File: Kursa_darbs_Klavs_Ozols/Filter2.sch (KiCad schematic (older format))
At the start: 11 parts, among them U1 TL074

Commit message: Shii ir kursa darba 3. iteraacija
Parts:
- C15, C16, C17, C18: footprint (none) -> Capacitors_THT:C_Axial_L5.1mm_D3.1mm_P10.00mm_Horizontal
- R10, R11, R12, R7, R8, R9: footprint (none) -> Resistors_THT:R_Axial_DIN0309_L9.0mm_D3.2mm_P5.08mm_Vertical
- U1: footprint (none) -> TL074:DIL14
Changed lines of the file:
@@
 F 0 "U1" H 3450 2900 50  0000 L CNN
 F 1 "TL074" H 3450 2500 50  0000 L CNN
-F 2 "" H 3400 2800 50  0001 C CNN
+F 2 "TL074:DIL14" H 3400 2800 50  0001 C CNN
 F 3 "" H 3500 2900 50  0001 C CNN
 	3    3450 2700
@@
 F 0 "U1" H 5600 2900 50  0000 L CNN
 F 1 "TL074" H 5600 2500 50  0000 L CNN
-F 2 "" H 5550 2800 50  0001 C CNN
+F 2 "TL074:DIL14" H 5550 2800 50  0001 C CNN
 F 3 "" H 5650 2900 50  0001 C CNN
 	4    5600 2700
@@
 F 0 "R7" V 2380 2800 50  0000 C CNN
 F 1 "6.8 k" V 2300 2800 50  0000 C CNN
-F 2 "" V 2230 2800 50  0001 C CNN
-F 3 "" H 2300 2800 50  0001 C CNN
+F 2 "Resistors_THT:R_Axial_DIN0309_L9.0mm_D3.2mm_P5.08mm_Vertical" V 2230 2800 50  0001 C CNN
+F 3 "https://eu.mouser.com/datasheet/2/219/MOS-16613.pdf" H 2300 2800 50  0001 C CNN
 	1    2300 2800
 	0    1    1    0
@@
 F 0 "R8" V 2630 2550 50  0000 C CNN
 F 1 "5.1 k" V 2550 2550 50  0000 C CNN
-F 2 "" V 2480 2550 50  0001 C CNN
-F 3 "" H 2550 2550 50  0001 C CNN
+F 2 "Resistors_THT:R_Axial_DIN0309_L9.0mm_D3.2mm_P5.08mm_Vertical" V 2480 2550 50  0001 C CNN
+F 3 "https://eu.mouser.com/datasheet/2/219/MOS-16613.pdf" H 2550 2550 50  0001 C CNN
 	1    2550 2550
 	1    0    0    -1
@@
 F 0 "R9" V 3030 3000 50  0000 C CNN
 F 1 "62k" V 2950 3000 50  0000 C CNN
-F 2 "" V 2880 3000 50  0001 C CNN
-F 3 "" H 2950 3000 50  0001 C CNN
+F 2 "Resistors_THT:R_Axial_DIN0309_L9.0mm_D3.2mm_P5.08mm_Vertical" V 2880 3000 50  0001 C CNN
+F 3 "https://eu.mouser.com/datasheet/2/219/MOS-16613.pdf" H 2950 3000 50  0001 C CNN
 	1    2950 3000
 	1    0    0    -1
@@
 F 0 "C18" H 4960 3270 50  0000 L CNN
 F 1 "220 nF" H 4960 3120 50  0000 L CNN
-F 2 "" H 4950 3200 50  0001 C CNN
-F 3 "" H 4950 3200 50  0001 C CNN
+F 2 "Capacitors_THT:C_Axial_L5.1mm_D3.1mm_P10.00mm_Horizontal" H 4950 3200 50  0001 C CNN
+F 3 "https://eu.mouser.com/datasheet/2/212/KEM_C1046_AXIAL_MOLDED_X7R-1145195.pdf" H 4950 3200 50  0001 C CNN
 	1    4950 3200
 	0    1    1    0
@@
 F 0 "C16" H 2760 3320 50  0000 L CNN
 F 1 "220 nF" H 2760 3170 50  0000 L CNN
-F 2 "" H 2750 3250 50  0001 C CNN
-F 3 "" H 2750 3250 50  0001 C CNN
+F 2 "Capacitors_THT:C_Axial_L5.1mm_D3.1mm_P10.00mm_Horizontal" H 2750 3250 50  0001 C CNN
+F 3 "https://eu.mouser.com/datasheet/2/212/KEM_C1046_AXIAL_MOLDED_X7R-1145195.pdf" H 2750 3250 50  0001 C CNN
 	1    2750 3250
 	0    1    1    0
@@
 F 0 "C15" H 2760 2870 50  0000 L CNN
 F 1 "220 nF" H 2760 2720 50  0000 L CNN
-F 2 "" H 2750 2800 50  0001 C CNN
-F 3 "" H 2750 2800 50  0001 C CNN
+F 2 "Capacitors_THT:C_Axial_L5.1mm_D3.1mm_P10.00mm_Horizontal" H 2750 2800 50  0001 C CNN
+F 3 "https://eu.mouser.com/datasheet/2/212/KEM_C1046_AXIAL_MOLDED_X7R-1145195.pdf" H 2750 2800 50  0001 C CNN
 	1    2750 2800
 	0    1    1    0
@@
 F 0 "R10" V 4330 2700 50  0000 C CNN
 F 1 "6.8 k" V 4250 2700 50  0000 C CNN
-F 2 "" V 4180 2700 50  0001 C CNN
-F 3 "" H 4250 2700 50  0001 C CNN
+F 2 "Resistors_THT:R_Axial_DIN0309_L9.0mm_D3.2mm_P5.08mm_Vertical" V 4180 2700 50  0001 C CNN
+F 3 "https://eu.mouser.com/datasheet/2/219/MOS-16613.pdf" H 4250 2700 50  0001 C CNN
 	1    4250 2700
 	0    1    1    0
@@
 F 0 "C17" H 4960 2870 50  0000 L CNN
 F 1 "220 nF" H 4960 2720 50  0000 L CNN
-F 2 "" H 4950 2800 50  0001 C CNN
-F 3 "" H 4950 2800 50  0001 C CNN
+F 2 "Capacitors_THT:C_Axial_L5.1mm_D3.1mm_P10.00mm_Horizontal" H 4950 2800 50  0001 C CNN
+F 3 "https://eu.mouser.com/datasheet/2/212/KEM_C1046_AXIAL_MOLDED_X7R-1145195.pdf" H 4950 2800 50  0001 C CNN
 	1    4950 2800
 	0    1    1    0
@@
 F 0 "R12" V 5280 3000 50  0000 C CNN
 F 1 "62k" V 5200 3000 50  0000 C CNN
-F 2 "" V 5130 3000 50  0001 C CNN
-F 3 "" H 5200 3000 50  0001 C CNN
+F 2 "Resistors_THT:R_Axial_DIN0309_L9.0mm_D3.2mm_P5.08mm_Vertical" V 5130 3000 50  0001 C CNN
+F 3 "https://eu.mouser.com/datasheet/2/219/MOS-16613.pdf" H 5200 3000 50  0001 C CNN
 	1    5200 3000
 	1    0    0    -1
@@
 F 0 "R11" V 4730 2450 50  0000 C CNN
 F 1 "5.1 k" V 4650 2450 50  0000 C CNN
-F 2 "" V 4580 2450 50  0001 C CNN
-F 3 "" H 4650 2450 50  0001 C CNN
+F 2 "Resistors_THT:R_Axial_DIN0309_L9.0mm_D3.2mm_P5.08mm_Vertical" V 4580 2450 50  0001 C CNN
+F 3 "https://eu.mouser.com/datasheet/2/219/MOS-16613.pdf" H 4650 2450 50  0001 C CNN
 	1    4650 2450
 	0    1    1    0

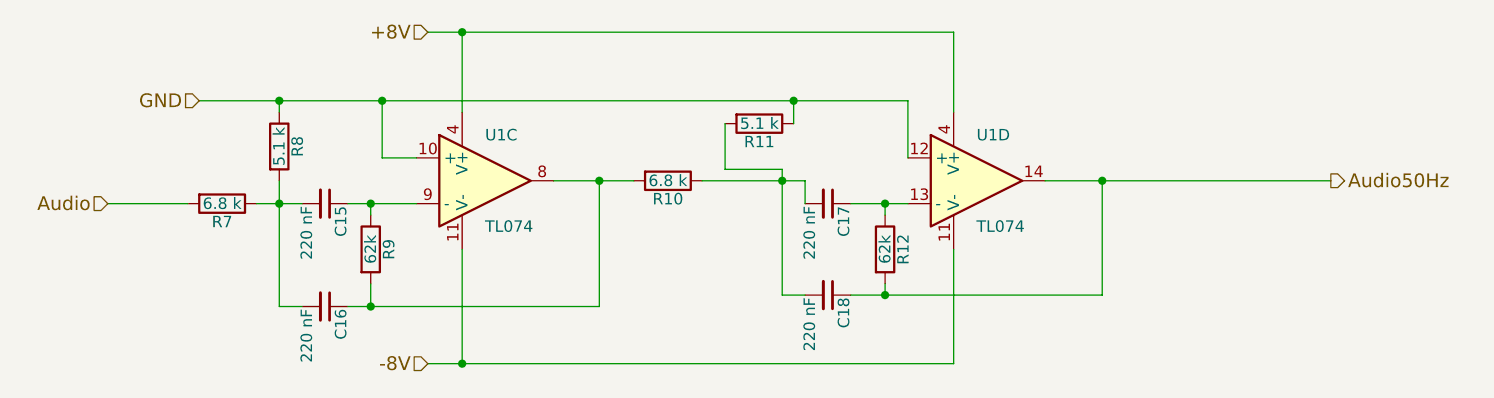
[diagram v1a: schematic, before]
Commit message: Shiii ir 5. iteraacija manai platei - layouts
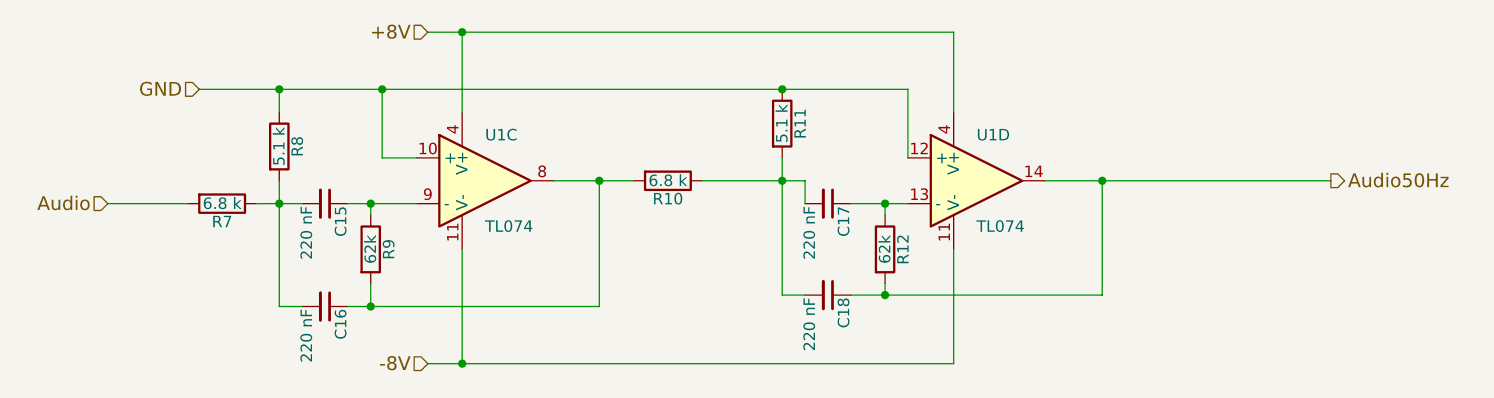
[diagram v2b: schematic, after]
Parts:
- C15, C16, C17, C18: footprint Capacitors_THT:C_Axial_L5.1mm_D3.1mm_P10.00mm_Horizontal -> Capacitors_SMD:C_0805_HandSoldering
- R10, R11, R12, R7, R8, R9: footprint Resistors_THT:R_Axial_DIN0309_L9.0mm_D3.2mm_P5.08mm_Vertical -> Resistors_SMD:R_0805_HandSoldering
- U1: footprint TL074:DIL14 -> TL074:SO14
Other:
- moved on the sheet: R11
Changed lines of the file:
@@
 EESchema Schematic File Version 2
+LIBS:Kursa_darbs_Klavs_Ozols-rescue
 LIBS:power
 LIBS:device
@@
 F 0 "U1" H 3450 2900 50  0000 L CNN
 F 1 "TL074" H 3450 2500 50  0000 L CNN
-F 2 "TL074:DIL14" H 3400 2800 50  0001 C CNN
+F 2 "TL074:SO14" H 3400 2800 50  0001 C CNN
 F 3 "" H 3500 2900 50  0001 C CNN
 	3    3450 2700
@@
 F 0 "U1" H 5600 2900 50  0000 L CNN
 F 1 "TL074" H 5600 2500 50  0000 L CNN
-F 2 "TL074:DIL14" H 5550 2800 50  0001 C CNN
+F 2 "TL074:SO14" H 5550 2800 50  0001 C CNN
 F 3 "" H 5650 2900 50  0001 C CNN
 	4    5600 2700
@@
 Text HLabel 3200 3500 0    60   Input ~ 0
 -8V
-Text HLabel 2200 2350 0    60   Input ~ 0
+Text HLabel 2200 2300 0    60   Input ~ 0
 GND
 $Comp
@@
 F 0 "R7" V 2380 2800 50  0000 C CNN
 F 1 "6.8 k" V 2300 2800 50  0000 C CNN
-F 2 "Resistors_THT:R_Axial_DIN0309_L9.0mm_D3.2mm_P5.08mm_Vertical" V 2230 2800 50  0001 C CNN
-F 3 "https://eu.mouser.com/datasheet/2/219/MOS-16613.pdf" H 2300 2800 50  0001 C CNN
+F 2 "Resistors_SMD:R_0805_HandSoldering" V 2230 2800 50  0001 C CNN
+F 3 "https://eu.mouser.com/datasheet/2/219/RN73-11994.pdf" H 2300 2800 50  0001 C CNN
 	1    2300 2800
 	0    1    1    0
@@
 F 0 "R8" V 2630 2550 50  0000 C CNN
 F 1 "5.1 k" V 2550 2550 50  0000 C CNN
-F 2 "Resistors_THT:R_Axial_DIN0309_L9.0mm_D3.2mm_P5.08mm_Vertical" V 2480 2550 50  0001 C CNN
-F 3 "https://eu.mouser.com/datasheet/2/219/MOS-16613.pdf" H 2550 2550 50  0001 C CNN
+F 2 "Resistors_SMD:R_0805_HandSoldering" V 2480 2550 50  0001 C CNN
+F 3 "https://eu.mouser.com/datasheet/2/219/RN73-11994.pdf" H 2550 2550 50  0001 C CNN
 	1    2550 2550
 	1    0    0    -1
@@
 F 0 "R9" V 3030 3000 50  0000 C CNN
 F 1 "62k" V 2950 3000 50  0000 C CNN
-F 2 "Resistors_THT:R_Axial_DIN0309_L9.0mm_D3.2mm_P5.08mm_Vertical" V 2880 3000 50  0001 C CNN
-F 3 "https://eu.mouser.com/datasheet/2/219/MOS-16613.pdf" H 2950 3000 50  0001 C CNN
+F 2 "Resistors_SMD:R_0805_HandSoldering" V 2880 3000 50  0001 C CNN
+F 3 "https://eu.mouser.com/datasheet/2/219/RN73-11994.pdf" H 2950 3000 50  0001 C CNN
 	1    2950 3000
 	1    0    0    -1
@@
 F 0 "C18" H 4960 3270 50  0000 L CNN
 F 1 "220 nF" H 4960 3120 50  0000 L CNN
-F 2 "Capacitors_THT:C_Axial_L5.1mm_D3.1mm_P10.00mm_Horizontal" H 4950 3200 50  0001 C CNN
-F 3 "https://eu.mouser.com/datasheet/2/212/KEM_C1046_AXIAL_MOLDED_X7R-1145195.pdf" H 4950 3200 50  0001 C CNN
+F 2 "Capacitors_SMD:C_0805_HandSoldering" H 4950 3200 50  0001 C CNN
+F 3 "https://eu.mouser.com/datasheet/2/427/vjcommercialseries-222796.pdf" H 4950 3200 50  0001 C CNN
 	1    4950 3200
 	0    1    1    0
@@
 F 0 "C16" H 2760 3320 50  0000 L CNN
 F 1 "220 nF" H 2760 3170 50  0000 L CNN
-F 2 "Capacitors_THT:C_Axial_L5.1mm_D3.1mm_P10.00mm_Horizontal" H 2750 3250 50  0001 C CNN
-F 3 "https://eu.mouser.com/datasheet/2/212/KEM_C1046_AXIAL_MOLDED_X7R-1145195.pdf" H 2750 3250 50  0001 C CNN
+F 2 "Capacitors_SMD:C_0805_HandSoldering" H 2750 3250 50  0001 C CNN
+F 3 "https://eu.mouser.com/datasheet/2/427/vjcommercialseries-222796.pdf" H 2750 3250 50  0001 C CNN
 	1    2750 3250
 	0    1    1    0
@@
 F 0 "C15" H 2760 2870 50  0000 L CNN
 F 1 "220 nF" H 2760 2720 50  0000 L CNN
-F 2 "Capacitors_THT:C_Axial_L5.1mm_D3.1mm_P10.00mm_Horizontal" H 2750 2800 50  0001 C CNN
-F 3 "https://eu.mouser.com/datasheet/2/212/KEM_C1046_AXIAL_MOLDED_X7R-1145195.pdf" H 2750 2800 50  0001 C CNN
+F 2 "Capacitors_SMD:C_0805_HandSoldering" H 2750 2800 50  0001 C CNN
+F 3 "https://eu.mouser.com/datasheet/2/427/vjcommercialseries-222796.pdf" H 2750 2800 50  0001 C CNN
 	1    2750 2800
 	0    1    1    0
@@
 F 0 "R10" V 4330 2700 50  0000 C CNN
 F 1 "6.8 k" V 4250 2700 50  0000 C CNN
-F 2 "Resistors_THT:R_Axial_DIN0309_L9.0mm_D3.2mm_P5.08mm_Vertical" V 4180 2700 50  0001 C CNN
-F 3 "https://eu.mouser.com/datasheet/2/219/MOS-16613.pdf" H 4250 2700 50  0001 C CNN
+F 2 "Resistors_SMD:R_0805_HandSoldering" V 4180 2700 50  0001 C CNN
+F 3 "https://eu.mouser.com/datasheet/2/219/RN73-11994.pdf" H 4250 2700 50  0001 C CNN
 	1    4250 2700
 	0    1    1    0
@@
 F 0 "C17" H 4960 2870 50  0000 L CNN
 F 1 "220 nF" H 4960 2720 50  0000 L CNN
-F 2 "Capacitors_THT:C_Axial_L5.1mm_D3.1mm_P10.00mm_Horizontal" H 4950 2800 50  0001 C CNN
-F 3 "https://eu.mouser.com/datasheet/2/212/KEM_C1046_AXIAL_MOLDED_X7R-1145195.pdf" H 4950 2800 50  0001 C CNN
+F 2 "Capacitors_SMD:C_0805_HandSoldering" H 4950 2800 50  0001 C CNN
+F 3 "https://eu.mouser.com/datasheet/2/427/vjcommercialseries-222796.pdf" H 4950 2800 50  0001 C CNN
 	1    4950 2800
 	0    1    1    0
@@
 F 0 "R12" V 5280 3000 50  0000 C CNN
 F 1 "62k" V 5200 3000 50  0000 C CNN
-F 2 "Resistors_THT:R_Axial_DIN0309_L9.0mm_D3.2mm_P5.08mm_Vertical" V 5130 3000 50  0001 C CNN
-F 3 "https://eu.mouser.com/datasheet/2/219/MOS-16613.pdf" H 5200 3000 50  0001 C CNN
+F 2 "Resistors_SMD:R_0805_HandSoldering" V 5130 3000 50  0001 C CNN
+F 3 "https://eu.mouser.com/datasheet/2/219/RN73-11994.pdf" H 5200 3000 50  0001 C CNN
 	1    5200 3000
 	1    0    0    -1
@@
 L R R11
 U 1 1 5B003CC0
-P 4650 2450
-F 0 "R11" V 4730 2450 50  0000 C CNN
-F 1 "5.1 k" V 4650 2450 50  0000 C CNN
-F 2 "Resistors_THT:R_Axial_DIN0309_L9.0mm_D3.2mm_P5.08mm_Vertical" V 4580 2450 50  0001 C CNN
-F 3 "https://eu.mouser.com/datasheet/2/219/MOS-16613.pdf" H 4650 2450 50  0001 C CNN
-	1    4650 2450
-	0    1    1    0
+P 4750 2450
+F 0 "R11" V 4830 2450 50  0000 C CNN
+F 1 "5.1 k" V 4750 2450 50  0000 C CNN
+F 2 "Resistors_SMD:R_0805_HandSoldering" V 4680 2450 50  0001 C CNN
+F 3 "https://eu.mouser.com/datasheet/2/219/MOS-16613.pdf" H 4750 2450 50  0001 C CNN
+	1    4750 2450
+	1    0    0    -1
 $EndComp
 Text HLabel 7150 2700 2    60   Output ~ 0
@@
 	2150 2800 1800 2800
 Wire Wire Line
-	3150 2600 3000 2600
-Wire Wire Line
-	3000 2600 3000 2350
-Wire Wire Line
-	2200 2350 5300 2350
-Wire Wire Line
-	2550 2400 2550 2350
-Connection ~ 2550 2350
+	3000 2600 3150 2600
+Wire Wire Line
+	3000 2300 3000 2600
+Wire Wire Line
+	2550 2300 2550 2400
 Wire Wire Line
 	2450 2800 2650 2800
@@
 Connection ~ 4750 2700
 Wire Wire Line
-	4750 2650 4750 3200
+	4750 2600 4750 3200
 Wire Wire Line
 	4750 3200 4850 3200
@@
 Connection ~ 5200 3200
 Connection ~ 6150 2700
-Connection ~ 3000 2350
-Wire Wire Line
-	5300 2350 5300 2600
+Wire Wire Line
+	5300 2300 5300 2600
 Wire Wire Line
 	3200 2050 5500 2050
@@
 Connection ~ 3350 3500
 Wire Wire Line
-	4800 2350 4800 2450
-Connection ~ 4800 2350
-Wire Wire Line
-	4500 2450 4500 2650
-Wire Wire Line
-	4500 2650 4750 2650
+	2200 2300 5300 2300
+Connection ~ 4750 2300
+Connection ~ 3000 2300
+Connection ~ 2550 2300
 $EndSCHEMATC
